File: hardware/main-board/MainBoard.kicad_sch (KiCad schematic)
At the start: 9 parts, among them U0 TL071, U1 TL071, U13 TL081, U2 TL071, U3 TL071, U5 STM32F091RCTx

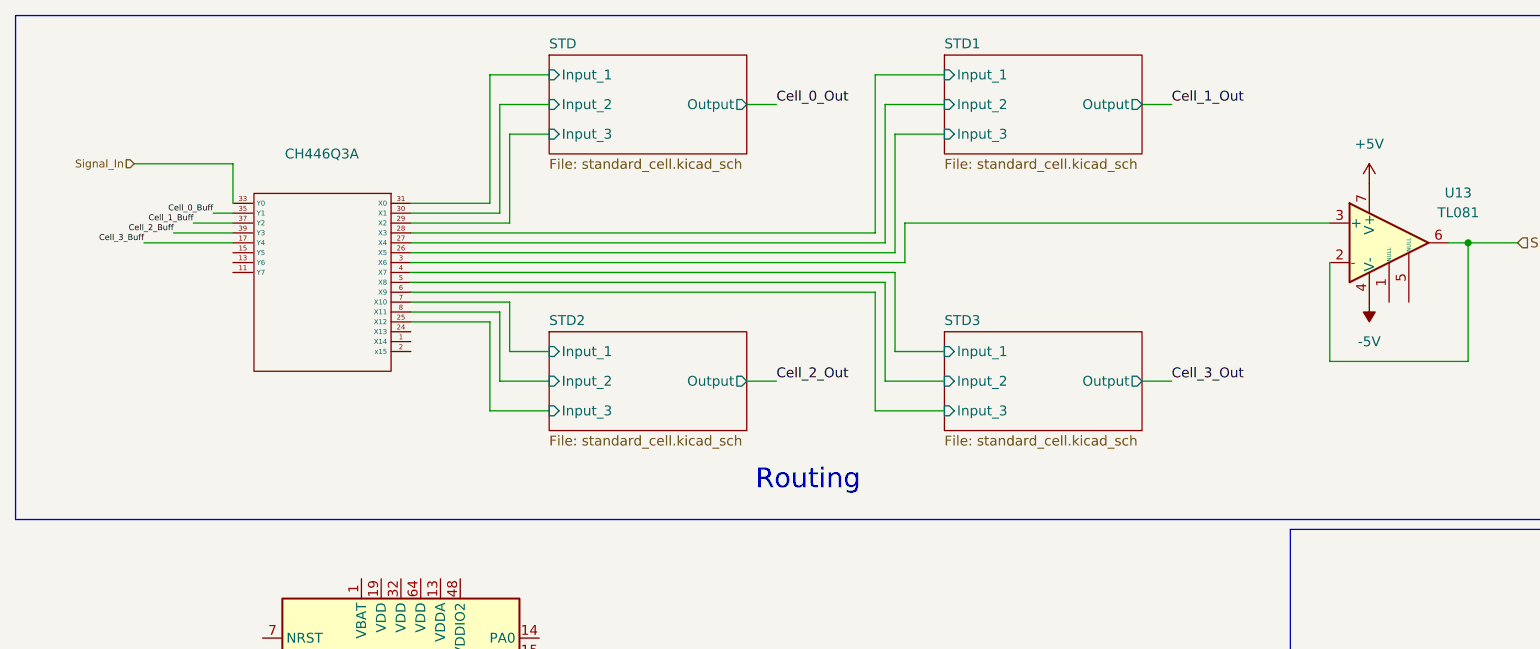
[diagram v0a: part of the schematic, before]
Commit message: Big Changes in the Schematic World
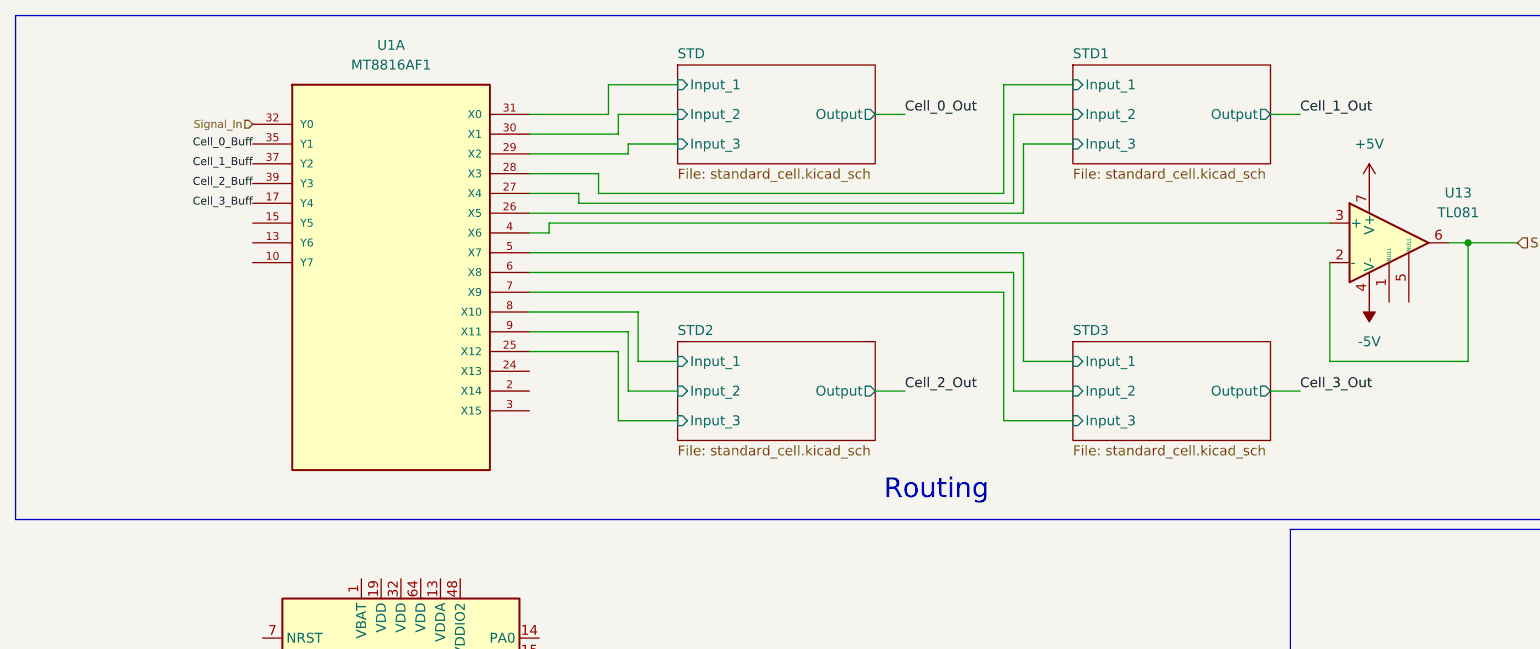
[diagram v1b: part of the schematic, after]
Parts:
- removed unit 1 of CH446Q3
- added U1: MT8816AF1, MT8816AF1:QFP80P1200X1200X120-44N, symbol SeniorDesign:MT8816AF1
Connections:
- net Cell_0_Buff: now also U1.35 (Y1)
- net Cell_1_Buff: now also U1.37 (Y2)
- net Cell_2_Buff: now also U1.39 (Y3)
- net Cell_3_Buff: now also U1.17 (Y4)
- net STD/Input_1: now also U1.31 (X0)
- net STD/Input_2: now also U1.30 (X1)
- net STD/Input_3: now also U1.29 (X2)
- net STD1/Input_1: now also U1.28 (X3)
- net STD1/Input_2: now also U1.27 (X4)
- net STD1/Input_3: now also U1.26 (X5)
- net STD2/Input_1: now also U1.8 (X10)
- net STD2/Input_2: now also U1.9 (X11)
- net STD2/Input_3: now also U1.25 (X12)
- net STD3/Input_1: now also U1.5 (X7)
- net STD3/Input_2: now also U1.6 (X8)
- net STD3/Input_3: now also U1.7 (X9)
- net Signal_In: now also U1.32 (Y0)
- net at U13.3 (+): now also U1.4 (X6)
